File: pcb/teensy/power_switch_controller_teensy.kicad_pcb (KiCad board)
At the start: 2 copper layers, 77.5 x 40.6 mm, 23 parts, among them P1 PWR_JACK_2.5x5.5_SMD_RA, P2 HEADER_01X03_SMD_RA, P3 HEADER_01X03_SMD_RA, P4 HEADER_01X03_SMD_RA, P5 BNC_DOUBLE_RA, P6 HEADER_01X02_SMD_RA, P7 HEADER_01X02_SMD_RA, SW1 KT_SWITCH

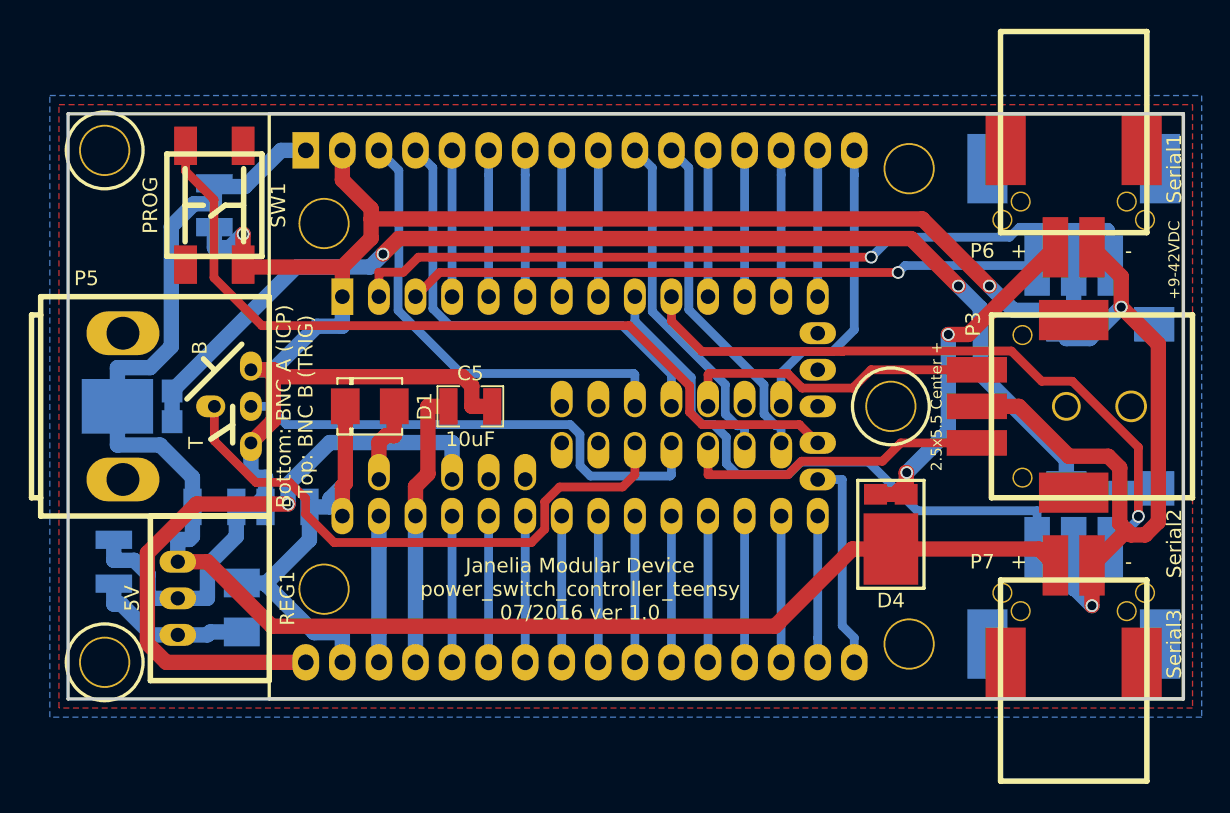
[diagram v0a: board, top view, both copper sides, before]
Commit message: More progress towards v1.0.
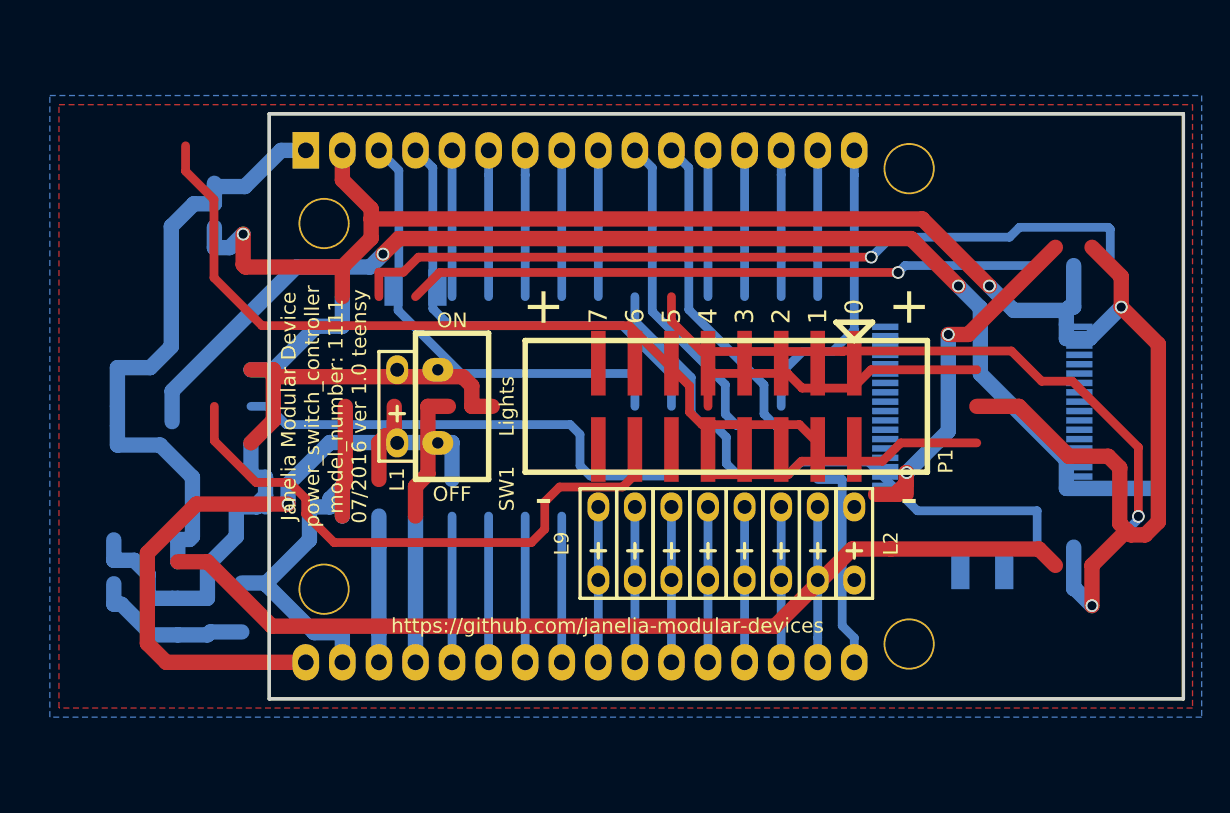
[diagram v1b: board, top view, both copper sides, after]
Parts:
- removed C3, C4, C5: 10uF, power_switch_controller_teensy:SM1210
- removed D1, D2: diode_schottky_15V_1A, power_switch_controller_teensy:DO-214BA
- removed D3, D4: diode_schottky_45V_10A, power_switch_controller_teensy:CFP15
- removed MNT_HOLE1, MNT_HOLE2, MNT_HOLE3: MNT_HOLE, power_switch_controller_teensy:MNT_HOLE
- removed P2, P3, P4: HEADER_01X03_SMD_RA, power_switch_controller_teensy:Header_3_Pin_SMD_RA
- removed P5: BNC_DOUBLE_RA, power_switch_controller_teensy:BNC_DOUBLE
- removed P6, P7: HEADER_01X02_SMD_RA, power_switch_controller_teensy:Header_2_Pin_SMD_RA
- removed REG1: CONV_DC_DC_5V_1A, power_switch_controller_teensy:DC_DC_CONV_R78C
- removed TEENSY1: TEENSY_3_2, power_switch_controller_teensy:TEENSY_3
- added L1: LED_24V, power_switch_controller_teensy:LED_555-3XXX, F.Cu at (82.5, 99.7)
- added L2: LED_24V, power_switch_controller_teensy:LED_555-3XXX, F.Cu at (114.3, 109.2)
- added L3: LED_24V, power_switch_controller_teensy:LED_555-3XXX, F.Cu at (111.8, 109.2)
- added L4: LED_24V, power_switch_controller_teensy:LED_555-3XXX, F.Cu at (109.2, 109.2)
- added L5: LED_24V, power_switch_controller_teensy:LED_555-3XXX, F.Cu at (106.7, 109.2)
- added L6: LED_24V, power_switch_controller_teensy:LED_555-3XXX, F.Cu at (104.1, 109.2)
- added L7: LED_24V, power_switch_controller_teensy:LED_555-3XXX, F.Cu at (101.6, 109.2)
- added L8: LED_24V, power_switch_controller_teensy:LED_555-3XXX, F.Cu at (99.1, 109.2)
- added L9: LED_24V, power_switch_controller_teensy:LED_555-3XXX, F.Cu at (96.5, 109.2)
- added U1: TLE7230R, power_switch_controller_teensy:PG-DSO-36, B.Cu at (123.2, 99.7)
- C2: value 10uF -> 0.1uF
- MDT1: value MODULAR_DEVICE_TEENSY -> MODULAR_DEVICE_TEENSY_MALE
- P1: value PWR_JACK_2.5x5.5_SMD_RA -> HEADER_02X08_SMD; footprint power_switch_controller_teensy:DCJACK_2PIN_HIGHCURRENT_SMD_RA -> power_switch_controller_teensy:HEADER_02x08_SMD; moved to F.Cu
- SW1: value KT_SWITCH -> SPST_SLIDE_AS; footprint power_switch_controller_teensy:KT_SWITCH -> power_switch_controller_teensy:SPST_SLIDE_AS
- moved C2 60.3 mm to (123.2, 111.1), turned to 0 degrees
- moved P1 26.7 mm to (105.4, 99.7)
- moved SW1 21.6 mm to (86.4, 99.7), turned to 0 degrees
- moved C1 20.7 mm to (83.8, 91.4), turned to 180 degrees
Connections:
- C2 pad 1: +5V -> VEE
- MDT1 pad 10: /D10 -> /CS
- MDT1 pad 11: /D11 -> /MOSI
- MDT1 pad 12: /D12 -> /MISO
- MDT1 pad 13: /D13 -> /SCK
- MDT1 pad 14: /D14 -> (no net)
- MDT1 pad 15: /D15 -> (no net)
- MDT1 pad 16: /D16 -> (no net)
- MDT1 pad 17: /D17 -> (no net)
- MDT1 pad 18: /D18 -> (no net)
- MDT1 pad 19: /D19 -> (no net)
- MDT1 pad 2: /D2 -> /RESET
- MDT1 pad 20: /D20 -> (no net)
- MDT1 pad 21: /D21 -> (no net)
- MDT1 pad 22: /D22 -> (no net)
- MDT1 pad 23: /D23 -> (no net)
- MDT1 pad 24: /D24 -> (no net)
- MDT1 pad 25: /D25 -> (no net)
- MDT1 pad 28: /D28 -> (no net)
- MDT1 pad 29: /D29 -> (no net)
- MDT1 pad 3: /D3 -> /PWM
- MDT1 pad 30: /D30 -> (no net)
- MDT1 pad 3V3: /3V3 -> (no net)
- MDT1 pad 4: /D4 -> (no net)
- MDT1 pad 5: /D5 -> (no net)
- MDT1 pad 6: /D6 -> (no net)
- MDT1 pad 9: /D9 -> (no net)
- MDT1 pad AGND: /AGND -> (no net)
- MDT1 pad AREF: /AREF -> (no net)
- MDT1 pad DAC: /DAC -> (no net)
- P1 pad 1: VAA -> VDD
- P1 pad 2: GND -> /OUT0
- P1 pad 3: (no net) -> VDD
- SW1 pad 1: (no net) -> VDD
- SW1 pad 3: GND -> /LED_PWR
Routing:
- net (no net): track 0.00 -> 570.8 mm, vias 0 -> 4
- net /OUT3: track 0.00 -> 89.8 mm, vias 0 -> 2
- net VAA: track 85.8 -> 0.00 mm, vias 2 -> 0
- net /OUT4: track 0.00 -> 73.9 mm
- net /PROG: track 57.7 -> 0.00 mm
- net /RX1: track 56.4 -> 0.00 mm, vias 1 -> 0
- net /LED_PWR: track 0.00 -> 51.4 mm, vias 0 -> 1
- net /OUT6: track 0.00 -> 50.6 mm
- net /AREF: track 45.5 -> 0.00 mm, vias 1 -> 0
- net /TX3: track 45.5 -> 0.00 mm, vias 1 -> 0
- net /TX1: track 44.1 -> 0.00 mm, vias 1 -> 0
- net /RX3: track 40.9 -> 0.00 mm
- net /BNC_A: track 40.4 -> 0.00 mm
- net /BNC_B: track 34.7 -> 0.00 mm
- net /D24: track 32.2 -> 0.00 mm
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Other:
- board size 77.5 x 40.6 mm -> 63.5 x 40.6 mm
- board text added: "0"
- board text added: "1"
- board text added: "2"
- board text added: "3"
- board text added: "4"
- board text added: "5"
- board text added: "6"
- board text added: "7"
- board text added: "Janelia Modular Device power_switch_controller model_number: 1111 07/2016 ver 1.0 teensy"
- board text added: "Lights"
- board text added: "https://github.com/janelia-modular-devices"
- board text removed: "+9-42VDC"
- board text removed: "2.5x5.5 Center +"
- board text removed: "5V"
- board text removed: "Janelia Modular Device power_switch_controller_teensy 07/2016 ver 1.0"
- board text removed: "Serial1"
- board text removed: "Serial2"
- board text removed: "Serial3"
